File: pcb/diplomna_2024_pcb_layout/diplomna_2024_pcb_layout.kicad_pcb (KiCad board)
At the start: 4 copper layers, 95 x 95 mm, 15 parts

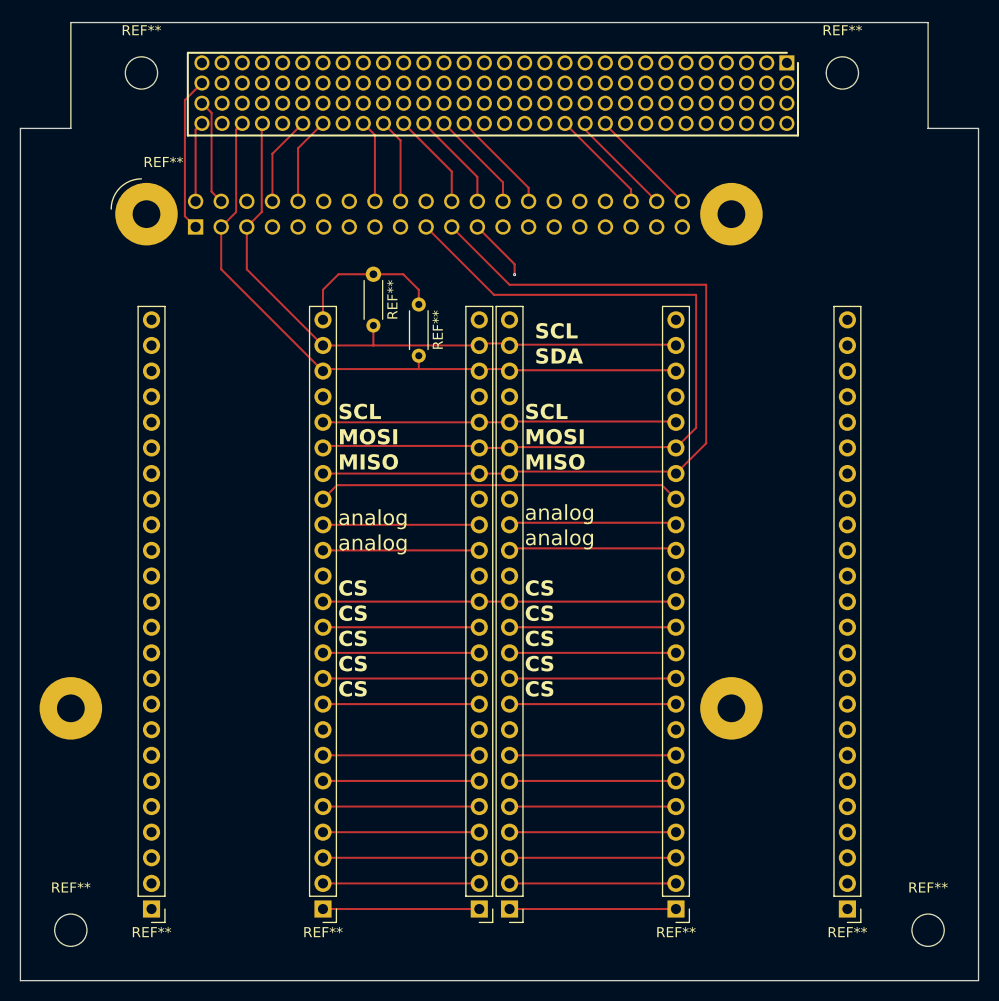
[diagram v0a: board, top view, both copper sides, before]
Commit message: pc design updates
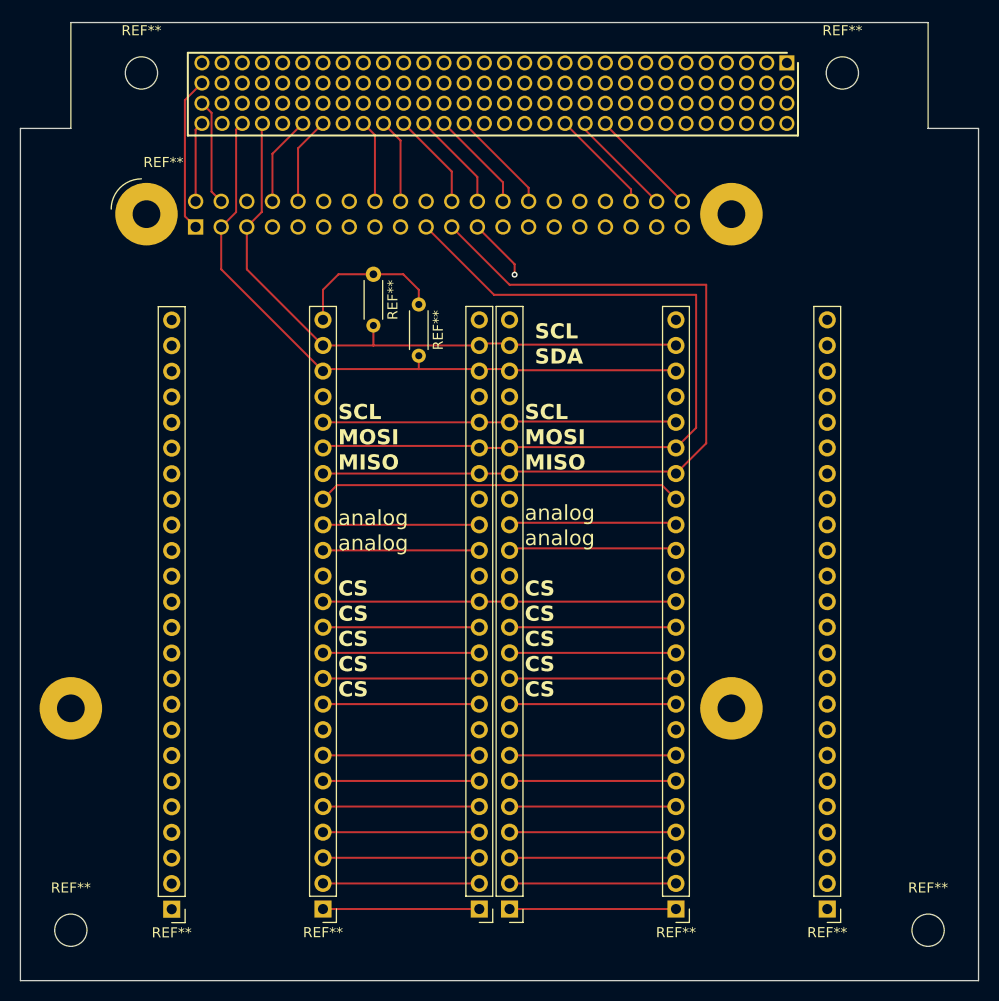
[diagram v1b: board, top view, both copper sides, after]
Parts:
- moved REF** 2.00 mm to (171.0, 138.4)
- moved REF** 2.00 mm to (236.0, 138.4)
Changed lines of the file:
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@@
 			(drillshape 0)
 			(scaleselection 1)
-			(outputdirectory "./")
+			(outputdirectory "v3/")
 		)
 	)
@@
 	(footprint "Connector_PinHeader_2.54mm:PinHeader_1x24_P2.54mm_Vertical"
 		(layer "F.Cu")
-		(at 238 138.4 180)
+		(at 236 138.4 180)
 		(descr "Through hole straight pin header, 1x24, 2.54mm pitch, single row")
 		(tags "Through hole pin header THT 1x24 2.54mm single row")
@@
 	(footprint "Connector_PinHeader_2.54mm:PinHeader_1x24_P2.54mm_Vertical"
 		(layer "F.Cu")
-		(at 169 138.4 180)
+		(at 171 138.42 180)
 		(descr "Through hole straight pin header, 1x24, 2.54mm pitch, single row")
 		(tags "Through hole pin header THT 1x24 2.54mm single row")
@@
 		(net 9)
 	)
-	(via micro
+	(via
 		(at 205 75.5)
-		(size 0.3)
-		(drill 0.1)
-		(layers "F.Cu" "In2.Cu")
+		(size 0.6)
+		(drill 0.3)
+		(layers "F.Cu" "B.Cu")
 		(free yes)
 		(net 9)
